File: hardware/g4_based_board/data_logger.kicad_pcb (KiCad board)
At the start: 4 copper layers, 100 x 100 mm, 132 parts, among them J1 Conn_01x07_Socket, J12 Screw_Terminal_01x04, J13 Conn_01x09_Pin, J2 Conn_02x07_Odd_Even, J3 Conn_01x07_Socket, J4 Conn_ARM_SWD_TagConnect_TC203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, J40 Conn_01x07_Socket, J43 Conn_01x06, J5 Screw_Terminal_01x03, J6 Conn_01x04, J7 Conn_01x05_Socket, J8 USB_C_Receptacle_USB2.0, J9 Micro_SD_Card_Det1, Q1 NPN, Q2 NPN, Q5 NMOS, SW1 RESET, SW2 SW_SPDT, SW3 DOWN, SW7 UP, SW8 ENTER, SW9 WAKE, U1 STM32G431R6Tx, U2 MCP9804_MSOP, U3 MCP3428x-xST, U4 TL074, U6 tps2117, U7 AZ1117-3.3, Y1 8MHZ, 18PF

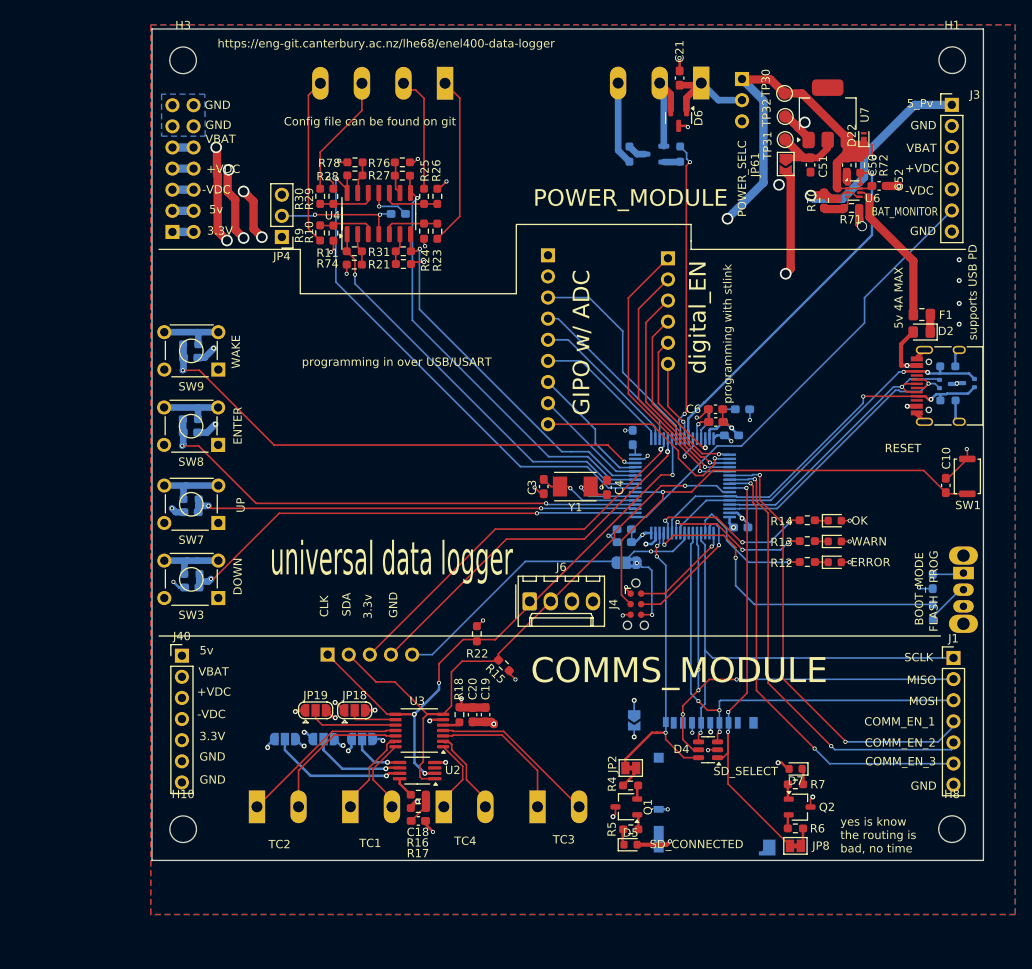
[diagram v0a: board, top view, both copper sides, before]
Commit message: auto updated
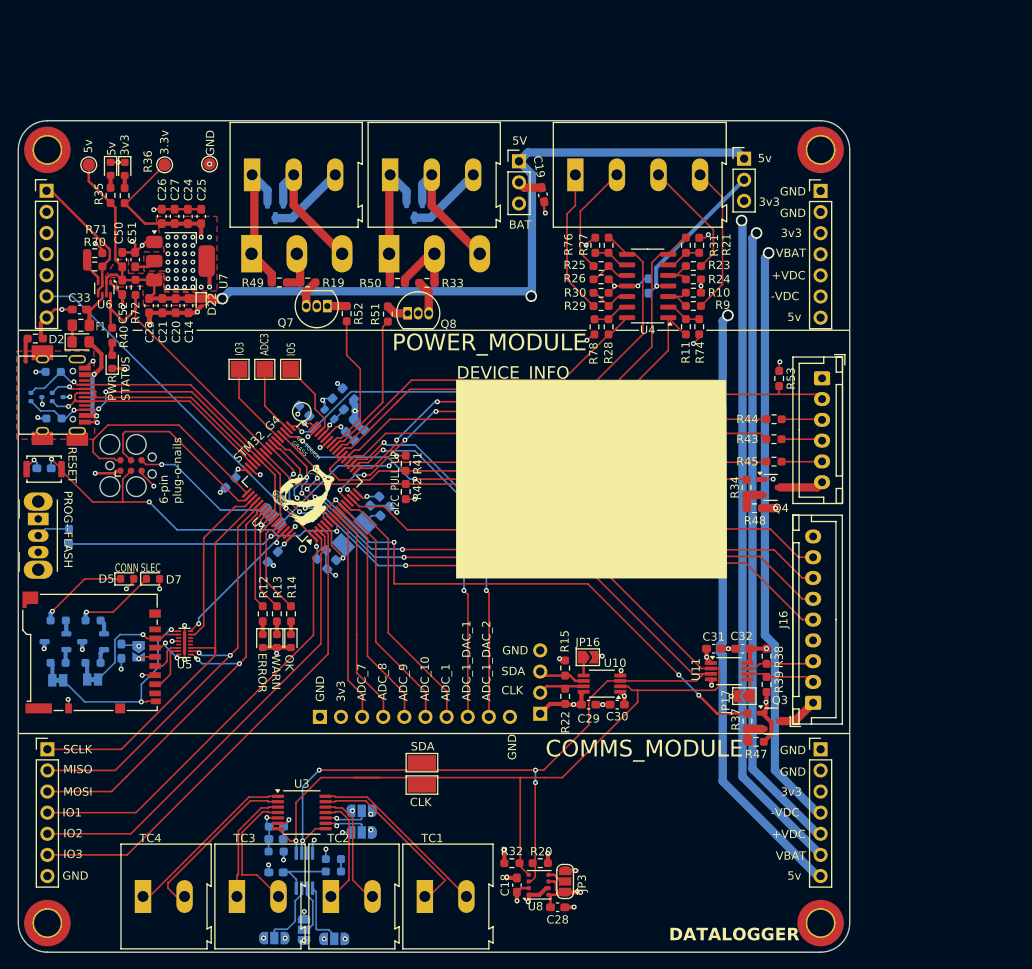
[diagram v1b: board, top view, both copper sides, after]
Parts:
- removed C53, C54, C55, C56: C, Capacitor_SMD:C_0603_1608Metric_Pad1.08x0.95mm_HandSolder
- removed D4: SP0505BAHT, Package_TO_SOT_SMD:SOT-23-6
- removed the G*** at (190.9, 133.5)
- removed the G*** at (169.9, 102.5)
- removed H10, H8: MountingHole, MountingHole:MountingHole_3.2mm_M3
- removed J13: Conn_01x09_Pin, Connector_PinHeader_2.54mm:PinHeader_1x09_P2.54mm_Vertical
- removed J43: Conn_01x06, Connector_PinHeader_2.54mm:PinHeader_1x06_P2.54mm_Vertical
- removed JP15, JP18, JP19: ~, Jumper:SolderJumper-3_P1.3mm_Open_RoundedPad1.0x1.5mm
- removed JP61: Jumper_2_Open, Jumper:SolderJumper-2_P1.3mm_Open_TrianglePad1.0x1.5mm
- removed R73, R75, R77, R79: R, Resistor_SMD:R_0603_1608Metric_Pad0.98x0.95mm_HandSolder
- removed SW3: DOWN, Button_Switch_THT:SW_TH_Tactile_Omron_B3F-10xx
- removed SW7: UP, Button_Switch_THT:SW_TH_Tactile_Omron_B3F-10xx
- removed SW8: ENTER, Button_Switch_THT:SW_TH_Tactile_Omron_B3F-10xx
- removed SW9: WAKE, Button_Switch_THT:SW_TH_Tactile_Omron_B3F-10xx
- added C14: 1u, Capacitor_SMD:C_0603_1608Metric_Pad1.08x0.95mm_HandSolder, F.Cu at (110.5, 81.2)
- added C15: 0.1u, Capacitor_SMD:C_0603_1608Metric_Pad1.08x0.95mm_HandSolder, B.Cu at (121.0, 149.4)
- added C16: 0.1u, Capacitor_SMD:C_0603_1608Metric_Pad1.08x0.95mm_HandSolder, B.Cu at (121.0, 145.4)
- added C17: 10u, Capacitor_SMD:C_0603_1608Metric_Pad1.08x0.95mm_HandSolder, B.Cu at (121.0, 143.9)
- added C23: 1u, Capacitor_SMD:C_0603_1608Metric_Pad1.08x0.95mm_HandSolder, F.Cu at (105.7, 81.2)
- added C24: 1u, Capacitor_SMD:C_0603_1608Metric_Pad1.08x0.95mm_HandSolder, F.Cu at (110.4, 70.5)
- added C25: 1u, Capacitor_SMD:C_0603_1608Metric_Pad1.08x0.95mm_HandSolder, F.Cu at (112.0, 70.5)
- added C26: 1u, Capacitor_SMD:C_0603_1608Metric_Pad1.08x0.95mm_HandSolder, F.Cu at (107.3, 70.5)
- added C27: 1u, Capacitor_SMD:C_0603_1608Metric_Pad1.08x0.95mm_HandSolder, F.Cu at (108.8, 70.5)
- added C28: 100n, Capacitor_SMD:C_0603_1608Metric_Pad1.08x0.95mm_HandSolder, F.Cu at (154.9, 153.6)
- added C29: 100n, Capacitor_SMD:C_0603_1608Metric_Pad1.08x0.95mm_HandSolder, F.Cu at (158.6, 129.2)
- added C30: 100n, Capacitor_SMD:C_0603_1608Metric_Pad1.08x0.95mm_HandSolder, F.Cu at (162.0, 129.2)
- added C31: 100n, Capacitor_SMD:C_0603_1608Metric_Pad1.08x0.95mm_HandSolder, F.Cu at (173.6, 122.5)
- added C32: 100n, Capacitor_SMD:C_0603_1608Metric_Pad1.08x0.95mm_HandSolder, F.Cu at (177.1, 122.5)
- added C33: 10u, Capacitor_SMD:C_0603_1608Metric_Pad1.08x0.95mm_HandSolder, F.Cu at (97.4, 81.7)
- added D12: SP0502BAHT, Package_TO_SOT_SMD:SOT-23, B.Cu at (137.6, 69.7)
- added D13: LED, LED_SMD:LED_0603_1608Metric, F.Cu at (101.1, 64.8)
- added D14: LED, LED_SMD:LED_0603_1608Metric, F.Cu at (102.8, 64.8)
- added D15: LED, LED_SMD:LED_0603_1608Metric, F.Cu at (101.3, 88.0)
- added G***: LOGO, frogs:frog_smaller, F.Cu at (124.7, 103.6)
- added H2: MountingHole_Pad, MountingHole:MountingHole_3.2mm_M3_DIN965_Pad_TopOnly, F.Cu at (186.5, 62.5)
- added H4: MountingHole_Pad, MountingHole:MountingHole_3.2mm_M3_DIN965_Pad_TopOnly, F.Cu at (186.5, 155.5)
- added J11: Conn_01x06_Pin, Connector_JST:JST_XH_B6B-XH-A_1x06_P2.50mm_Vertical, F.Cu at (186.7, 90.0)
- added J15: Screw_Terminal_01x03, TerminalBlock:TerminalBlock_Altech_AK300-3_P5.00mm, F.Cu at (134.7, 65.5)
- added J16: Conn_01x09, Connector_JST:JST_XH_B9B-XH-A_1x09_P2.50mm_Vertical, F.Cu at (185.6, 129.0)
- added JP10: ~, Jumper:SolderJumper-3_P1.3mm_Open_RoundedPad1.0x1.5mm, B.Cu at (128.0, 157.4)
- added JP11: ~, Jumper:SolderJumper-3_P1.3mm_Open_RoundedPad1.0x1.5mm, B.Cu at (131.3, 144.6)
- added JP12: ~, Jumper:SolderJumper-3_P1.3mm_Open_RoundedPad1.0x1.5mm, B.Cu at (131.3, 142.0)
- added JP6: power_select, Connector_PinHeader_2.54mm:PinHeader_1x03_P2.54mm_Vertical, F.Cu at (150.2, 63.9)
- added JP7: ~, Jumper:SolderJumper-3_P1.3mm_Open_RoundedPad1.0x1.5mm, B.Cu at (120.8, 157.3)
- added JP9: ~, Jumper:SolderJumper-3_P1.3mm_Open_RoundedPad1.0x1.5mm, B.Cu at (124.4, 156.3)
- added Q3: PMOS, Package_TO_SOT_SMD:SOT-23-3, F.Cu at (180.6, 131.2)
- added Q4: PMOS, Package_TO_SOT_SMD:SOT-23-3, F.Cu at (180.5, 103.1)
- added Q6: PMOS, Package_TO_SOT_THT:TO-247-3_Vertical, B.Cu at (134.6, 75.0)
- added Q7: 2N3904, Package_TO_SOT_THT:TO-92_Inline, F.Cu at (127.2, 81.3)
- added Q8: 2N3904, Package_TO_SOT_THT:TO-92_Inline, F.Cu at (136.8, 82.2)
- added R32: 4.7k, Resistor_SMD:R_0603_1608Metric_Pad0.98x0.95mm_HandSolder, F.Cu at (149.4, 148.3)
- added R33: 10, Resistor_SMD:R_0603_1608Metric_Pad0.98x0.95mm_HandSolder, F.Cu at (139.2, 78.5)
- added R34: 10, Resistor_SMD:R_0603_1608Metric_Pad0.98x0.95mm_HandSolder, F.Cu at (177.6, 103.1)
- added R35: R, Resistor_SMD:R_0603_1608Metric_Pad0.98x0.95mm_HandSolder, F.Cu at (101.1, 68.0)
- added R36: R, Resistor_SMD:R_0603_1608Metric_Pad0.98x0.95mm_HandSolder, F.Cu at (102.8, 68.0)
- added R37: 10, Resistor_SMD:R_0603_1608Metric_Pad0.98x0.95mm_HandSolder, F.Cu at (177.7, 131.2)
- added R38: 4.7k, Resistor_SMD:R_0603_1608Metric_Pad0.98x0.95mm_HandSolder, F.Cu at (180.0, 123.4)
- added R39: 4.7k, Resistor_SMD:R_0603_1608Metric_Pad0.98x0.95mm_HandSolder, F.Cu at (180.0, 126.8)
- added R40: R, Resistor_SMD:R_0603_1608Metric_Pad0.98x0.95mm_HandSolder, F.Cu at (101.3, 84.8)
- added R41: 4.7k, Resistor_SMD:R_0603_1608Metric_Pad0.98x0.95mm_HandSolder, F.Cu at (136.6, 100.2)
- added R42: 4.7k, Resistor_SMD:R_0603_1608Metric_Pad0.98x0.95mm_HandSolder, F.Cu at (136.6, 103.6)
- added R43: 0, Resistor_SMD:R_0603_1608Metric_Pad0.98x0.95mm_HandSolder, F.Cu at (180.9, 97.3)
- added R44: 0, Resistor_SMD:R_0603_1608Metric_Pad0.98x0.95mm_HandSolder, F.Cu at (180.9, 94.9)
- added R45: 0, Resistor_SMD:R_0603_1608Metric_Pad0.98x0.95mm_HandSolder, F.Cu at (180.9, 100.0)
- added R46: R, Resistor_SMD:R_0603_1608Metric_Pad0.98x0.95mm_HandSolder, F.Cu at (92.0, 85.2)
- added R47: 1k, Resistor_SMD:R_0603_1608Metric_Pad0.98x0.95mm_HandSolder, F.Cu at (178.8, 133.7)
- added R48: 1k, Resistor_SMD:R_0603_1608Metric_Pad0.98x0.95mm_HandSolder, F.Cu at (178.6, 105.6)
- added R49: 10k, Resistor_SMD:R_0603_1608Metric_Pad0.98x0.95mm_HandSolder, F.Cu at (121.4, 78.5)
- added R50: 10k, Resistor_SMD:R_0603_1608Metric_Pad0.98x0.95mm_HandSolder, F.Cu at (135.6, 78.5)
- added R51: 10k, Resistor_SMD:R_0603_1608Metric_Pad0.98x0.95mm_HandSolder, F.Cu at (134.4, 82.2)
- added R52: 10k, Resistor_SMD:R_0603_1608Metric_Pad0.98x0.95mm_HandSolder, F.Cu at (129.5, 82.2)
- added R53: 4.7k, Resistor_SMD:R_0603_1608Metric_Pad0.98x0.95mm_HandSolder, F.Cu at (181.5, 90.0)
- added TP1: TestPoint, TestPoint:TestPoint_Keystone_5015_Micro-Minature, F.Cu at (138.6, 136.2)
- added TP2: TestPoint, TestPoint:TestPoint_Keystone_5015_Micro-Minature, F.Cu at (138.6, 138.9)
- added TP4: TestPoint, TestPoint:TestPoint_Pad_2.0x2.0mm, F.Cu at (122.8, 88.9)
- added TP5: TestPoint, TestPoint:TestPoint_Pad_2.0x2.0mm, F.Cu at (119.7, 88.9)
- added TP6: TestPoint, TestPoint:TestPoint_Pad_2.0x2.0mm, F.Cu at (116.5, 88.9)
- added U10: TCA9800, Package_SO:VSSOP-8_3.0x3.0mm_P0.65mm, F.Cu at (160.2, 126.7)
- added U11: TCA9800, Package_SO:VSSOP-8_3.0x3.0mm_P0.65mm, F.Cu at (175.5, 125.2)
- added U5: CM1624, Package_DFN_QFN:OnSemi_UDFN-16-1EP_1.35x3.3mm_P0.4mm_EP0.4x2.8mm, F.Cu at (110.0, 121.8)
- added U8: BME680, Package_LGA:Bosch_LGA-8_3x3mm_P0.8mm_ClockwisePinNumbering, F.Cu at (152.6, 150.9)
- C10, C2, C3, C4, C6, D6, JP2, JP8, Q1, Q2, R16, R17, R18, R4, R5, R6, R7, U2, Y1: moved to B.Cu
- C18: value 0.1u -> 100n
- C19: value 0.1u -> 10u
- C20: value 10u -> 1u
- C21: value C -> 1u
- H1, H3: value MountingHole -> MountingHole_Pad; footprint MountingHole:MountingHole_3.2mm_M3 -> MountingHole:MountingHole_3.2mm_M3_DIN965_Pad_TopOnly
- J12, J5, J9, SW2, TC1, TC2, TC3, TC4, U1: moved to F.Cu
- J2: value Conn_02x07_Odd_Even -> Conn_01x07_Socket; footprint Connector_PinHeader_2.54mm:PinHeader_2x07_P2.54mm_Vertical -> Connector_PinHeader_2.54mm:PinHeader_1x07_P2.54mm_Vertical; moved to F.Cu
- J4: footprint Connector:Tag-Connect_TC2030-IDC-NL_2x03_P1.27mm_Vertical -> Connector:Tag-Connect_TC2030-IDC-FP_2x03_P1.27mm_Vertical
- J6: footprint Connector_Molex:Molex_KK-254_AE-6410-04A_1x04_P2.54mm_Vertical -> Connector_PinHeader_2.54mm:PinHeader_1x04_P2.54mm_Vertical; moved to B.Cu
- J7: value Conn_01x05_Socket -> Conn_01x10; footprint Connector_PinHeader_2.54mm:PinHeader_1x05_P2.54mm_Vertical -> Connector_PinHeader_2.54mm:PinHeader_1x10_P2.54mm_Vertical
- JP16, JP17: value ~ -> Jumper_2_Open; footprint Jumper:SolderJumper-3_P1.3mm_Open_RoundedPad1.0x1.5mm -> Jumper:SolderJumper-2_P1.3mm_Open_TrianglePad1.0x1.5mm; moved to F.Cu
- JP3: value power_select -> ~; footprint Connector_PinHeader_2.54mm:PinHeader_1x03_P2.54mm_Vertical -> Jumper:SolderJumper-3_P1.3mm_Open_RoundedPad1.0x1.5mm; moved to F.Cu
- Q5: value NMOS -> PMOS; footprint Package_TO_SOT_SMD:SOT-23-3 -> Package_TO_SOT_THT:TO-247-3_Vertical
- R19: value 1k -> 10; moved to F.Cu
- R20: value 1k -> 4.7k; moved to F.Cu
- R70: value 10k -> 16.9k
- R71: value 10k -> 5k
- moved D1 112.2 mm to (92.2, 92.2), turned to 0 degrees
- moved SW2 111.5 mm to (92.4, 106.9)
- moved SW1 111.1 mm to (93.1, 100.9), turned to 0 degrees
- moved J1 109.5 mm to (93.5, 134.6)
- moved J3 109.4 mm to (93.4, 67.4)
- moved H1 109.4 mm to (93.5, 62.5)
- moved C10 108.5 mm to (93.1, 100.8), turned to 0 degrees
- moved J8 108.2 mm to (94.0, 92.0), turned to -90 degrees
- moved R2 107.7 mm to (94.3, 94.8), turned to 180 degrees
- moved R3 107.7 mm to (94.2, 89.2), turned to 180 degrees
- moved D3 106.7 mm to (94.7, 92.2)
- moved H3 105.0 mm to (93.5, 155.5)
- moved R1 104.3 mm to (96.1, 109.0), turned to -90 degrees
- moved D2 101.2 mm to (97.5, 85.6), turned to 0 degrees
- moved F1 101.2 mm to (97.5, 83.6), turned to 180 degrees
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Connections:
- net /high_speed_digital/thermocouples/T1_+ renamed /high_speed_digital/T1_+
- net /high_speed_digital/thermocouples/T1_- renamed /high_speed_digital/T1_-
- net /high_speed_digital/thermocouples/T2_+ renamed /high_speed_digital/T2_+
- net /high_speed_digital/thermocouples/T2_- renamed /high_speed_digital/T2_-
- net /high_speed_digital/thermocouples/T3_+ renamed /high_speed_digital/T3_+
- net /high_speed_digital/thermocouples/T3_- renamed /high_speed_digital/T3_-
- net /high_speed_digital/thermocouples/T4_+ renamed /high_speed_digital/T4_+
- net /high_speed_digital/thermocouples/T4_- renamed /high_speed_digital/T4_-
- C1 pad 1: +3.3V -> /V_bat_monitor
- C18 pad 1: Net-(C18-Pad1) -> +3.3V
- C19 pad 1: +3.3V -> /power_amp/PWR
- C20 pad 1: +3.3V -> +5V
- C21 pad 1: Net-(J5-Pin_1) -> +5V
- C51 pad 1: Net-(JP61-A) -> +3.3V
- D6 pad 1: Net-(J5-Pin_1) -> /power_amp/PWR
- J2 pad 1: +3.3V -> GND
- J2 pad 2: +3.3V -> GND
- J2 pad 3: +5V -> +3.3V
- J2 pad 4: +5V -> -VDC
- J2 pad 5: -VDC -> +VDC
- J2 pad 6: -VDC -> +BATT
- J2 pad 7: +VDC -> +5V
- J40 pad 1: +5V -> GND
- J40 pad 2: +3.3V -> GND
- J40 pad 3: +BATT -> +3.3V
- J40 pad 4: +VDC -> +BATT
- J40 pad 5: -VDC -> +VDC
- J40 pad 6: GND -> -VDC
- J40 pad 7: GND -> +5V
- J5 pad 1: Net-(J5-Pin_1) -> /power_amp/PWR
- J6 pad 1: /high_speed_digital/I2C_CLK -> +3.3V
- J6 pad 2: /high_speed_digital/SDA -> Net-(J6-Pin_2)
- J6 pad 3: +3.3V -> Net-(J6-Pin_3)
- J7 pad 1: /high_speed_digital/I2C_CLK -> GND
- J7 pad 2: /high_speed_digital/SDA -> +3.3V
- J7 pad 3: /high_speed_digital/MISO -> /mcu/ADC-GPIO-PWM-7
- J7 pad 4: /high_speed_digital/MOSI -> /mcu/ADC-GPIO-PWM-8
- J7 pad 5: /high_speed_digital/SCLK -> /mcu/ADC-GPIO-PWM-9
- J8 pad S1: GND -> GNDS
- J9 pad 3: /interface/MOSI -> /interface/MOSI_SD
- J9 pad 7: /interface/MISO -> /interface/MISO_SD
- JP16 pad 1: GND -> Net-(JP16-A)
- JP16 pad 2: Net-(JP16-C) -> GND
- JP17 pad 1: GND -> Net-(JP17-A)
- JP17 pad 2: Net-(JP17-C) -> GND
- JP3 pad 1: +5V -> +3.3V
- JP3 pad 2: Net-(J5-Pin_1) -> Net-(JP3-C)
- JP3 pad 3: +BATT -> GND
- Q5 pad 1: Net-(J5-Pin_2) -> /power_amp/PWR
- Q5 pad 3: Net-(Q5-S) -> Net-(J5-Pin_2)
- R15 pad 2: /high_speed_digital/SDA -> Net-(J6-Pin_3)
- R16 pad 1: +3.3V -> Net-(R16-Pad1)
- R16 pad 2: Net-(C18-Pad1) -> Net-(U2-V_{DD})
- R17 pad 1: Net-(C18-Pad1) -> +3.3V
- R17 pad 2: Net-(U2-V_{DD}) -> Net-(R16-Pad1)
- R19 pad 2: /mcu/ADC-GPIO-PWM-11 -> Net-(Q7-C)
- R20 pad 1: Net-(Q5-S) -> +3.3V
- R20 pad 2: GND -> /high_speed_digital/SDA
- R22 pad 2: /high_speed_digital/I2C_CLK -> Net-(J6-Pin_2)
- R23 pad 2: /analog_in/SIG_IN_1 -> /analog_in/SIG_IN_4
- R29 pad 2: /analog_in/SIG_IN_4 -> /analog_in/SIG_IN_1
- TP31 pad 1: Net-(JP61-A) -> +3.3V
- U1 pad 10: /analog_in/ADC_3 -> /mcu/ADC-GPIO-PWM-9
- U1 pad 11: /analog_in/ADC_1 -> /mcu/ADC-GPIO-PWM-10
- U1 pad 13: /mcu/ADC-GPIO-PWM-2-DIFF1-2 -> /analog_in/ADC_2
- U1 pad 14: /interface/WAKE_BTN -> /high_speed_digital/BTN_1
- U1 pad 17: /mcu/ADC-GPIO-PWM-4 -> /analog_in/ADC_1
- U1 pad 2: /interface/DOWN_BTN -> /mcu/COMMS_EN_1
- U1 pad 23: /mcu/ADC-GPIO-PWM-12 -> /analog_in/ADC_3
- U1 pad 24: /mcu/ADC-GPIO-PWM-11 -> /analog_in/ADC_4
- U1 pad 25: /mcu/DIGITAL_IO_EN_4 -> /mcu/PWM_2
- U1 pad 26: /mcu/PWR_STATUS -> /mcu/PWM_1
- U1 pad 3: /interface/UP_BTN -> /mcu/COMMS_EN_2
- U1 pad 33: /mcu/DIGITAL_IO_EN_6 -> /high_speed_digital/CS
- U1 pad 35: /mcu/DIGITAL_IO_EN_1 -> /high_speed_digital/CAMERA_POWER_EN
- U1 pad 36: /mcu/DIGITAL_IO_EN_2 -> /high_speed_digital/HI_POWER_EN
- U1 pad 38: /mcu/COMMS_EN_1 -> /high_speed_digital/BTN_4
- U1 pad 39: /mcu/COMMS_EN_2 -> /high_speed_digital/BTN_2
- U1 pad 4: /interface/ENTER_BTN -> /mcu/COMMS_EN_3
- U1 pad 40: /mcu/COMMS_EN_3 -> /high_speed_digital/BTN_3
- U1 pad 41: /interface/SD_SELECT -> /mcu/PWR_STATUS
- U1 pad 51: /mcu/DEBUG_LED_1 -> /interface/SD_CARD_SELECT
- U1 pad 55: unconnected-(U1-PD2-Pad55) -> /mcu/DEBUG_LED_1
- U1 pad 8: /analog_in/ADC_4 -> /mcu/ADC-GPIO-PWM-7
- U1 pad 9: /analog_in/ADC_2 -> /mcu/ADC-GPIO-PWM-8
- U2 pad 1: /high_speed_digital/SDA -> /high_speed_digital/I2C_CLK
- U2 pad 2: /high_speed_digital/I2C_CLK -> /high_speed_digital/SDA
- U2 pad 5: Net-(JP17-C) -> Net-(JP10-C)
- U2 pad 6: Net-(JP16-C) -> Net-(JP9-C)
- U3 pad 7: /high_speed_digital/SDA -> /high_speed_digital/I2C_CLK
- U3 pad 8: /high_speed_digital/I2C_CLK -> /high_speed_digital/SDA
- U7 pad 2: Net-(JP61-A) -> +3.3V
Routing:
- net /high_speed_digital/BTN_3: track 0.00 -> 77.3 mm, vias 0 -> 6
- net /power_amp/PWR: track 0.00 -> 76.9 mm
- net /high_speed_digital/BTN_2: track 0.00 -> 76.3 mm, vias 0 -> 6
- net /high_speed_digital/HI_POWER_EN: track 0.00 -> 75.9 mm, vias 0 -> 6
- net /high_speed_digital/BTN_4: track 0.00 -> 74.8 mm, vias 0 -> 6
- net /high_speed_digital/I2C_CLK: track 71.8 -> 146.0 mm, vias 4 -> 1
- net /high_speed_digital/SDA: track 75.6 -> 146.6 mm, vias 1 -> 4
- net /high_speed_digital/CS: track 0.00 -> 68.4 mm, vias 0 -> 2
- net /interface/WAKE_BTN: track 62.3 -> 0.00 mm, vias 2 -> 0
- net /interface/ENTER_BTN: track 60.6 -> 0.00 mm, vias 2 -> 0
- net /high_speed_digital/BTN_1: track 0.00 -> 58.8 mm, vias 0 -> 2
- net /high_speed_digital/CAMERA_POWER_EN: track 0.00 -> 57.9 mm, vias 0 -> 4
- net /interface/DOWN_BTN: track 57.5 -> 0.00 mm, vias 2 -> 0
- net +5V: track 181.5 -> 236.6 mm, vias 1 -> 3
- net /interface/UP_BTN: track 54.3 -> 0.00 mm, vias 2 -> 0
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- added copper zone on F.Cu, net +3.3V
- added copper zone on In2.Cu, net +3.3V
- added copper zone on F.Cu, net +5V
- added copper zone on In1.Cu, net GND
- added copper zone on F.Cu, net GNDS
- removed copper zone on In1.Cu, net +3.3V
- removed copper zone on B.Cu, net GND
- removed copper zone on F.Cu, net GND
- removed copper zone on In2.Cu, net GND
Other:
- outline, holes or cut-outs redrawn
- board text added: "3v3"
- board text added: "5v_IN"
- board text added: "6-pin plug-o-nails"
- board text added: "ADC3"
- board text added: "ADC_1"
- board text added: "ADC_10"
- board text added: "ADC_1_DAC_1"
- board text added: "ADC_1_DAC_2"
- board text added: "ADC_7"
- board text added: "ADC_8"
- board text added: "ADC_9"
- board text added: "BAT"
- board text added: "BTN1"
- board text added: "BTN2"
- board text added: "BTN3"
- board text added: "BTN4"
- board text added: "CONN"
- board text added: "CS"
- board text added: "DATALOGGER"
- board text added: "DEVICE_INFO"
- board text added: "GO TOUCH GRASS"
- board text added: "I2C_PULL_UP"
- board text added: "IO1"
- board text added: "IO2"
- board text added: "IO3"
- board text added: "IO5"
- board text added: "PROG--FLASH"
- board text added: "PWR STATUS"
- board text added: "SLEC"
- board text added: "STM32_G4"
- board text added: "V_MONITOR"
- board text removed: "3.3V"
- board text removed: "5_Pv"
- board text removed: "5v 4A MAX"
- board text removed: "ADC-10"
- board text removed: "ADC-12"
- board text removed: "ADC-1_DIFF_1"
- board text removed: "ADC-2_DIFF_2"
- board text removed: "ADC-3"
- board text removed: "ADC-4"
- board text removed: "ADC-9"
- board text removed: "BAT_MONITOR"
- board text removed: "BOOT_MODE"
- board text removed: "COMM_EN_1"
- board text removed: "COMM_EN_2"
- board text removed: "COMM_EN_3"
- board text removed: "Config file can be found on git"
- board text removed: "DAC1"
- board text removed: "DAC2"
- board text removed: "DOWN"
- board text removed: "EN-1"
- board text removed: "EN-2"
- board text removed: "EN-3"
- board text removed: "EN-4"
- board text removed: "EN-5"
- board text removed: "EN-6"
- board text removed: "ENEL-400W-GROUP-E31"
- board text removed: "ENTER"
- board text removed: "FLASH"
- board text removed: "GIPO w/ ADC"
- board text removed: "ID: 72740637"
- board text removed: "LOGAN HENDERSON"
- board text removed: "M3 hole size"
- board text removed: "POWER_SELC"
- board text removed: "PROG"
- board text removed: "PWM-GND"
- board text removed: "PWR"
- board text removed: "SD CARD"
- board text removed: "SD_CONNECTED"
- board text removed: "SD_SELECT"
- board text removed: "SIG_1_IN"
- board text removed: "SIG_2_IN"
- board text removed: "SIG_3_IN"
- board text removed: "SIG_4_IN"
- board text removed: "STM32G431RBT6"
- board text removed: "TC1"
- board text removed: "TC2"
- board text removed: "TC3"
- board text removed: "TC4"
- board text removed: "UP"
- board text removed: "WAKE"
- board text removed: "digital_EN"
- board text removed: "programming in over USB/USART"
- board text removed: "programming with stlink"
- board text removed: "supports USB PD"
- board text removed: "universal data logger"
- board text removed: "yes is know the routing is bad, no time"
